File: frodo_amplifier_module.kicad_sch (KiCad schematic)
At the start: 35 parts, among them IC1 MCP3221A5T-I_OT, IC2 INA826AID, J1 Conn_01x01_Socket, J2 Conn_01x01_Socket, J3 Conn_01x01_Socket, J4 Conn_01x01_Socket, J5 Conn_01x01_Socket, J6 Conn_01x01_Socket, J7 Conn_01x01_Socket, J8 Conn_01x01_Socket, U1 MCP602, U2 MIC5504-3.3YM5

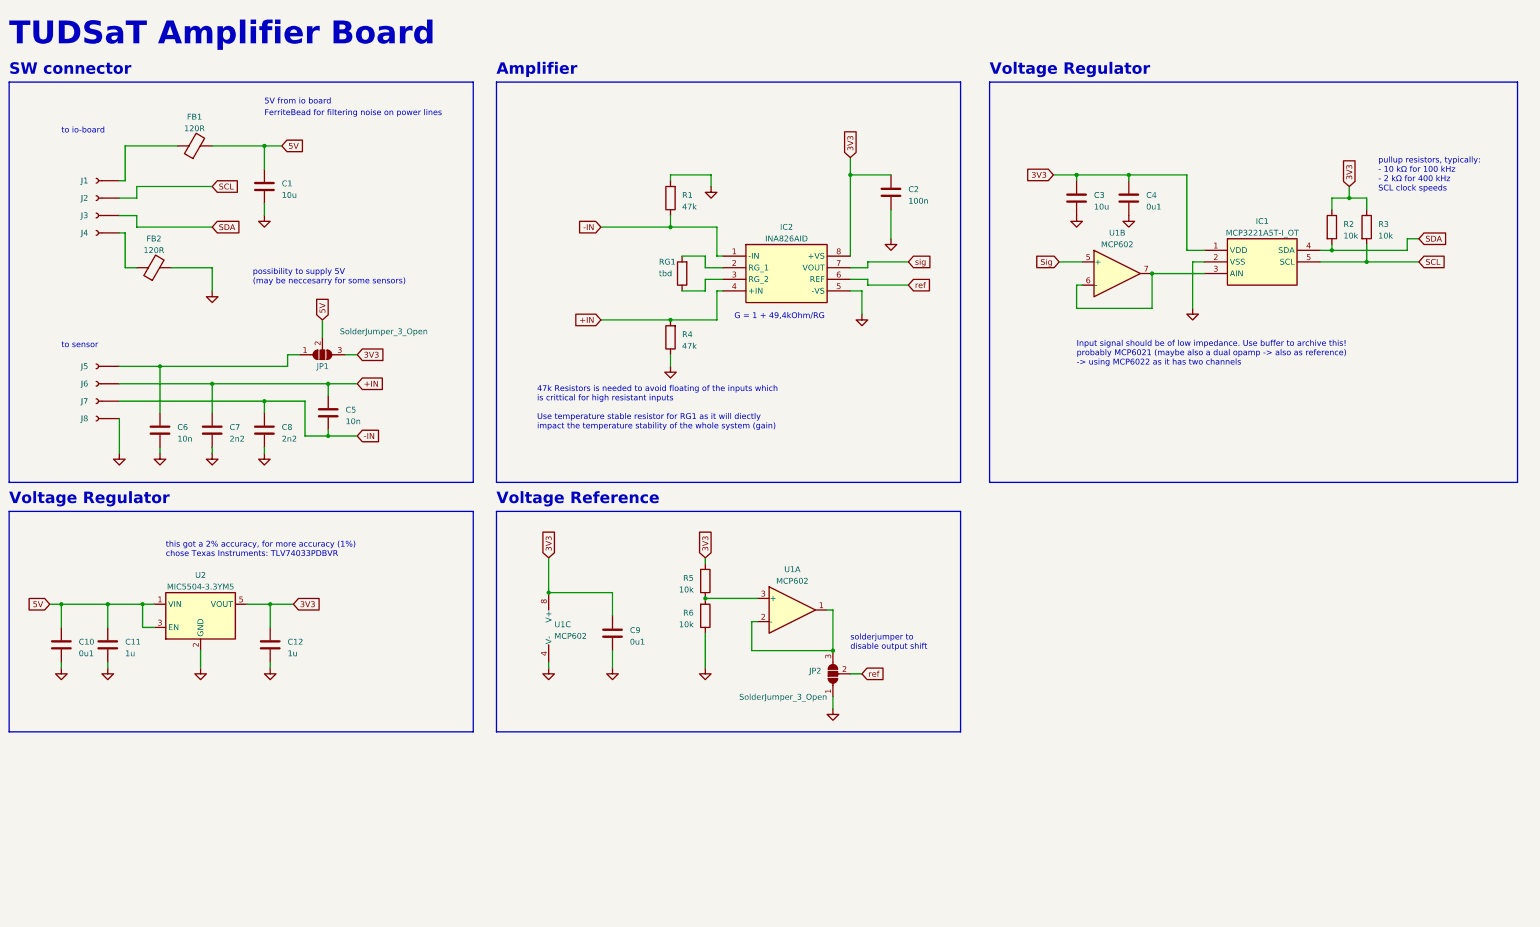
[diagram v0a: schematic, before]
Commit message: finished the scematics
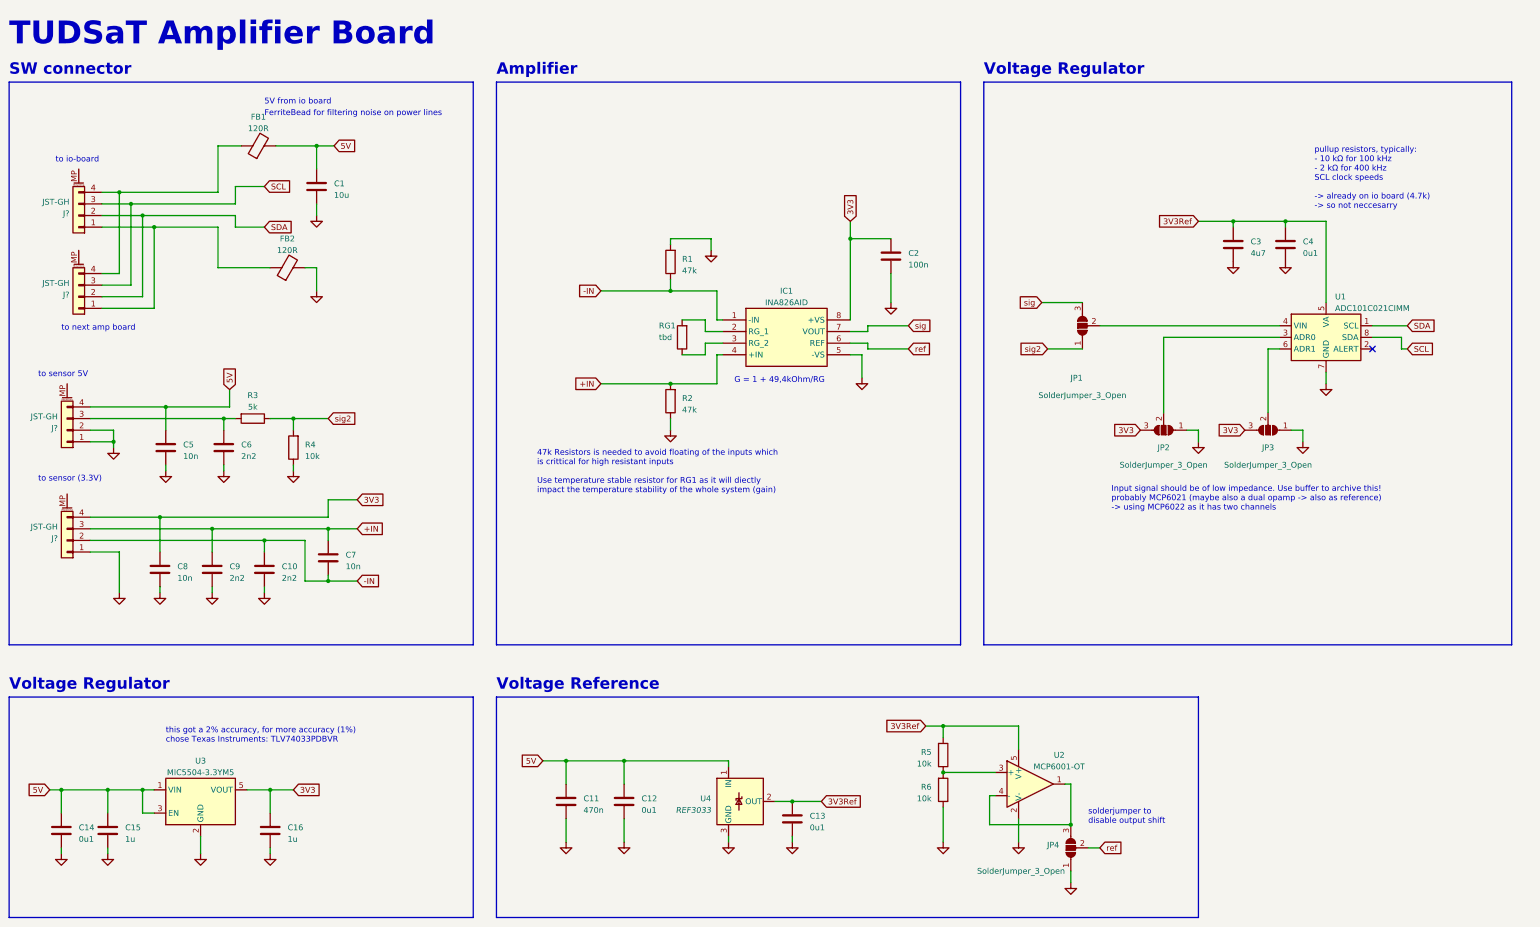
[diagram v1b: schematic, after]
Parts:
- removed C9: 0u1, Capacitor_SMD:C_0402_1005Metric, symbol Device:C
- removed IC1: MCP3221A5T-I_OT, Package_TO_SOT_SMD:SOT-23-5, symbol MCP3221A5T-I_OT:MCP3221A5T-I_OT
- removed J1, J2, J3, J4, J5, J6, J7, J8: Conn_01x01_Socket, Connector_Wire:SolderWirePad_1x01_SMD_1x2mm, symbol Connector:Conn_01x01_Socket
- removed R2: 10k, Resistor_SMD:R_0402_1005Metric, symbol Device:R
- removed U1: MCP602, Package_SO:SOIC-8-1EP_3.9x4.9mm_P1.27mm_EP2.29x3mm, symbol Amplifier_Operational:MCP602
- added C11: 470n, Capacitor_SMD:C_0402_1005Metric, symbol Device:C
- added C12, C13: 0u1, Capacitor_SMD:C_0402_1005Metric, symbol Device:C
- added C5: 10n, Capacitor_SMD:C_0402_1005Metric, symbol Device:C
- added C6: 2n2, Capacitor_SMD:C_0402_1005Metric, symbol Device:C
- added J? (x4): JST-GH, Connector_JST:JST_GH_BM04B-GHS-TBT_1x04-1MP_P1.25mm_Vertical, symbol Connector_Generic_MountingPin:Conn_01x04_MountingPin
- added JP2, JP3: SolderJumper_3_Open, Jumper:SolderJumper-3_P1.3mm_Open_RoundedPad1.0x1.5mm, symbol Jumper:SolderJumper_3_Open
- added R4: 10k, Resistor_SMD:R_0402_1005Metric_Pad0.72x0.64mm_HandSolder, symbol Device:R
- added U1: ADC101C021CIMM, Package_SO:SSOP-8_2.95x2.8mm_P0.65mm, symbol Analog_ADC:ADC101C021CIMM
- added U2: MCP6001-OT, Package_TO_SOT_SMD:SOT-23-5, symbol Amplifier_Operational:MCP6001-OT
- added U4: REF3033, Package_TO_SOT_SMD:SOT-23, symbol Reference_Voltage:REF3033
- C1: footprint Capacitor_SMD:C_0603_1608Metric -> Capacitor_SMD:C_0402_1005Metric
- C3: value 10u -> 4u7; footprint Capacitor_SMD:C_0603_1608Metric -> Capacitor_SMD:C_0402_1005Metric
- FB1, FB2: footprint Inductor_SMD:L_0603_1608Metric -> Inductor_SMD:L_0402_1005Metric
- IC1: renamed from IC2; footprint Package_SO:SOIC-8_3.9x4.9mm_P1.27mm -> Package_SON:WSON-8-1EP_3x3mm_P0.5mm_EP1.2x2mm
- JP1: footprint Jumper:SolderJumper-3_P1.3mm_Open_RoundedPad1.0x1.5mm_NumberLabels -> Jumper:SolderJumper-3_P1.3mm_Open_RoundedPad1.0x1.5mm
- R1: footprint Resistor_SMD:R_0402_1005Metric_Pad0.72x0.64mm_HandSolder -> Resistor_SMD:R_0402_1005Metric
- R3: value 10k -> 5k; footprint Resistor_SMD:R_0402_1005Metric -> Resistor_SMD:R_0402_1005Metric_Pad0.72x0.64mm_HandSolder
- RG1: footprint Resistor_SMD:R_0603_1608Metric_Pad0.98x0.95mm_HandSolder -> Resistor_SMD:R_0603_1608Metric
- renumbered C8 to C10, C10 to C14, C11 to C15, C12 to C16, C5 to C7, C6 to C8, C7 to C9, JP2 to JP4, R4 to R2, U2 to U3
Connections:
- net +IN: now also J?.3 (Pin_3)
- net -IN: now also J?.2 (Pin_2)
- net 3V3: now also C8.1, J?.4 (Pin_4), JP2.3 (B), JP3.3 (B); no longer C3.1, C4.1, JP1.3 (B), R3.1, R5.2
- net 5V: now also C11.1, C12.1, C5.1, J?.4 (Pin_4), U4.1 (IN); no longer JP1.2 (C)
- net GND: now also C11.2, C12.2, C13.2, C5.2, C6.2, J?.1 (Pin_1), J?.1 (Pin_1), J?.2 (Pin_2), JP2.1 (A), JP3.1 (A), R4.1, U1.7 (GND), U2.2 (V-), U4.3 (GND)
- net SCL: now also J?.3 (Pin_3), J?.3 (Pin_3), U1.8 (SDA); no longer R3.2
- net SDA: now also J?.2 (Pin_2), J?.2 (Pin_2), U1.1 (SCL)
- net sig: now also JP1.3 (B)
- net sig2: now reaches JP1.1 (A)
- net sig2: now also R3.1, R4.2; no longer C8.1
- net at FB2.1: now also J?.1 (Pin_1), J?.1 (Pin_1)
- net at R5.1, R6.2: now also U2.3 (+)
- net at JP4.3 (B): now also U2.1, U2.4 (-)
- net at FB1.1: now also J?.4 (Pin_4), J?.4 (Pin_4)
- new net: JP2.2 (C), U1.3 (ADR0)
- new net: JP1.2 (C), U1.4 (VIN)
- new net: JP3.2 (C), U1.6 (ADR1)
- new net: C6.1, J?.3 (Pin_3), R3.2
- new net 3V3Ref: C13.1, C3.1, C4.1, R5.2, U1.5 (VA), U2.5 (V+), U4.2 (OUT)
- no-connect marks 0 -> 1
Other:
- note added: "pullup resistors, typically: - 10 kΩ for 100 kHz - 2 kΩ for 400 kHz SCL clock speeds -> already on io board (4.7k) -> so not neccesarry"
- note added: "to next amp board"
- note added: "to sensor (3.3V)"
- note added: "to sensor 5V"
- note removed: "possibility to supply 5V (may be neccesarry for some sensors)"
- note removed: "pullup resistors, typically: - 10 kΩ for 100 kHz - 2 kΩ for 400 kHz SCL clock speeds"
- note removed: "to sensor"
- moved on the sheet: C1, C10, C14, C15, C16, C2, C3, C4, C7, C8, C9, FB1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
